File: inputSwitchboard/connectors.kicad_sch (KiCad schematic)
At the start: 0 parts

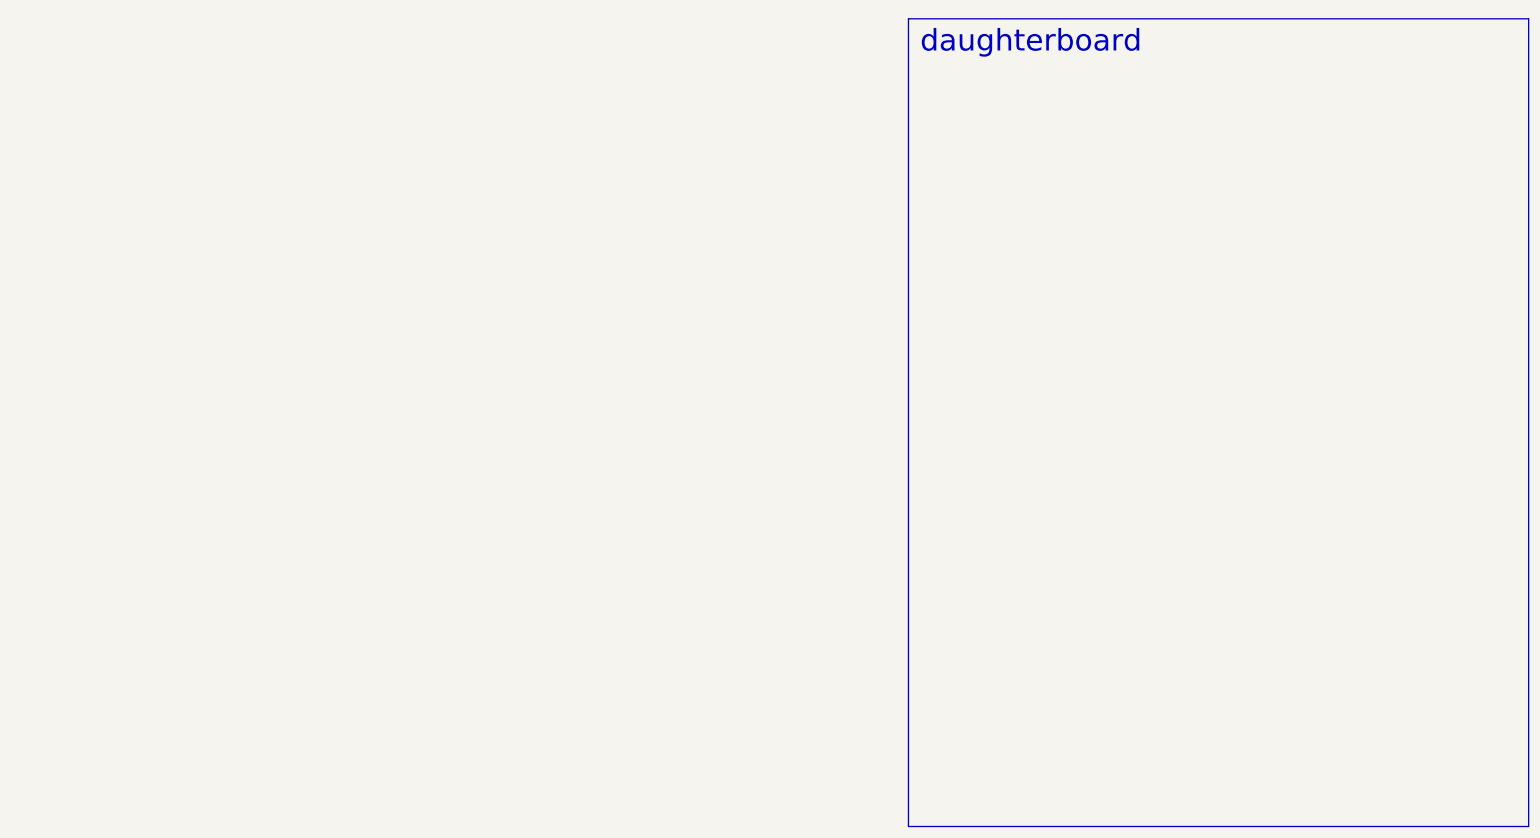
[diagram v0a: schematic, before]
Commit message: finished schematic
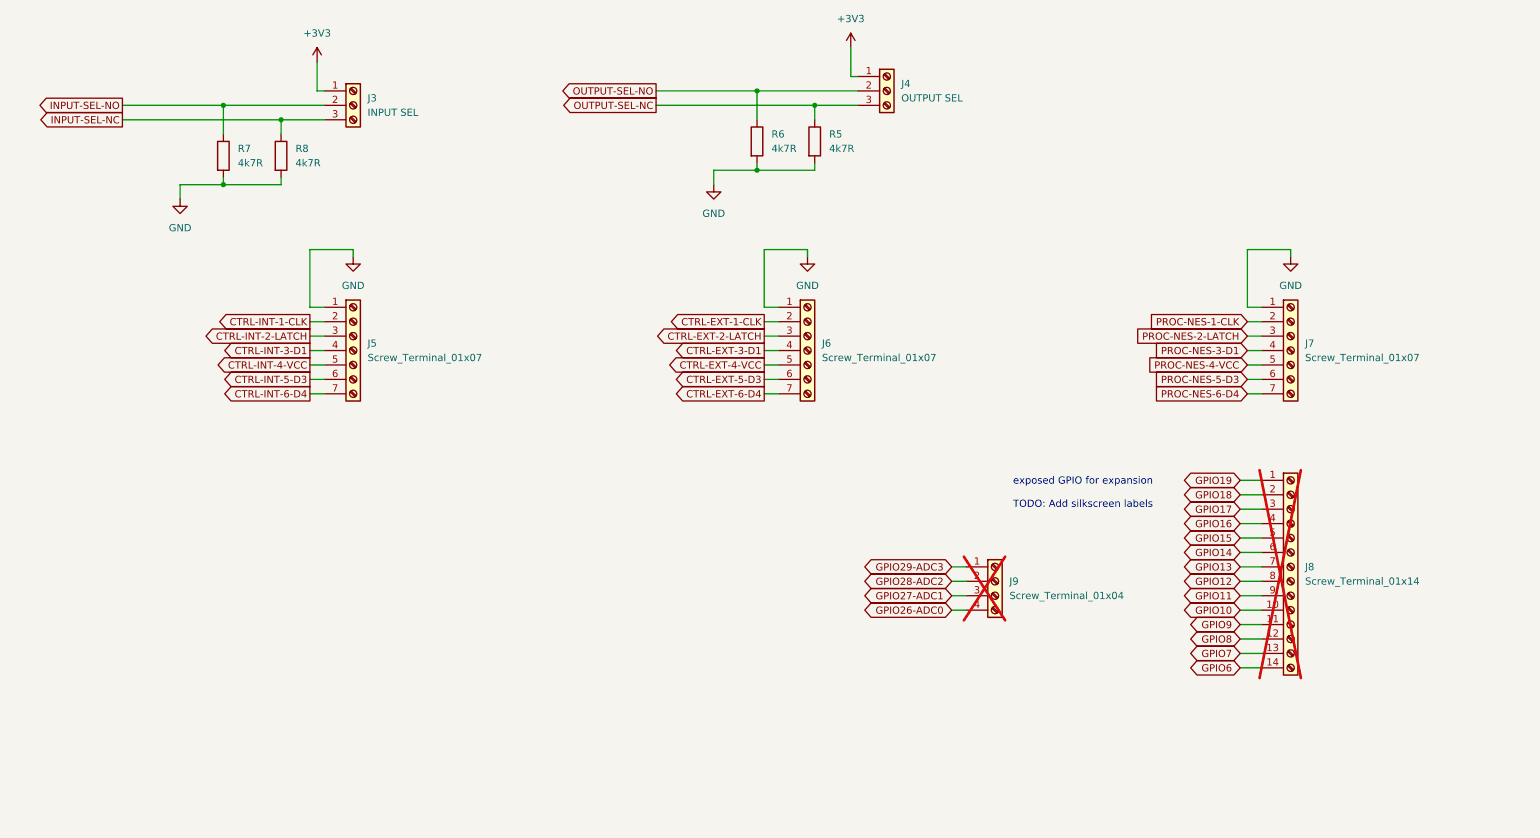
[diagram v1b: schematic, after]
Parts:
- added J3: INPUT SEL, TerminalBlock_Phoenix:TerminalBlock_Phoenix_MKDS-1,5-3-5.08_1x03_P5.08mm_Horizontal, symbol Connector:Screw_Terminal_01x03
- added J4: OUTPUT SEL, TerminalBlock_Phoenix:TerminalBlock_Phoenix_MKDS-1,5-3-5.08_1x03_P5.08mm_Horizontal, symbol Connector:Screw_Terminal_01x03
- added J5, J6, J7: Screw_Terminal_01x07, symbol Connector:Screw_Terminal_01x07
- added J8: Screw_Terminal_01x14, symbol Connector:Screw_Terminal_01x14
- added J9: Screw_Terminal_01x04, symbol Connector:Screw_Terminal_01x04
- added R5, R6, R7, R8: 4k7R, Resistor_SMD:R_0603_1608Metric, symbol Device:R
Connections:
- new net +3V3: J3.1 (Pin_1), J4.1 (Pin_1)
- new net CTRL-EXT-1-CLK: J6.2 (Pin_2)
- new net CTRL-EXT-2-LATCH: J6.3 (Pin_3)
- new net CTRL-EXT-3-D1: J6.4 (Pin_4)
- new net CTRL-EXT-4-VCC: J6.5 (Pin_5)
- new net CTRL-EXT-5-D3: J6.6 (Pin_6)
- new net CTRL-EXT-6-D4: J6.7 (Pin_7)
- new net CTRL-INT-1-CLK: J5.2 (Pin_2)
- new net CTRL-INT-2-LATCH: J5.3 (Pin_3)
- new net CTRL-INT-3-D1: J5.4 (Pin_4)
- new net CTRL-INT-4-VCC: J5.5 (Pin_5)
- new net CTRL-INT-5-D3: J5.6 (Pin_6)
- new net CTRL-INT-6-D4: J5.7 (Pin_7)
- new net GND: J5.1 (Pin_1), J6.1 (Pin_1), J7.1 (Pin_1), R5.2, R6.2, R7.2, R8.2
- new net GPIO10: J8.10 (Pin_10)
- new net GPIO11: J8.9 (Pin_9)
- new net GPIO12: J8.8 (Pin_8)
- new net GPIO13: J8.7 (Pin_7)
- new net GPIO14: J8.6 (Pin_6)
- new net GPIO15: J8.5 (Pin_5)
- new net GPIO16: J8.4 (Pin_4)
- new net GPIO17: J8.3 (Pin_3)
- new net GPIO18: J8.2 (Pin_2)
- new net GPIO19: J8.1 (Pin_1)
- new net GPIO26-ADC0: J9.4 (Pin_4)
- new net GPIO27-ADC1: J9.3 (Pin_3)
- new net GPIO28-ADC2: J9.2 (Pin_2)
- new net GPIO29-ADC3: J9.1 (Pin_1)
- new net GPIO6: J8.14 (Pin_14)
- new net GPIO7: J8.13 (Pin_13)
- new net GPIO8: J8.12 (Pin_12)
- new net GPIO9: J8.11 (Pin_11)
- new net INPUT-SEL-NC: J3.3 (Pin_3), R8.1
- new net INPUT-SEL-NO: J3.2 (Pin_2), R7.1
- new net OUTPUT-SEL-NC: J4.3 (Pin_3), R5.1
- new net OUTPUT-SEL-NO: J4.2 (Pin_2), R6.1
- new net PROC-NES-1-CLK: J7.2 (Pin_2)
- new net PROC-NES-2-LATCH: J7.3 (Pin_3)
- new net PROC-NES-3-D1: J7.4 (Pin_4)
- new net PROC-NES-4-VCC: J7.5 (Pin_5)
- new net PROC-NES-5-D3: J7.6 (Pin_6)
- new net PROC-NES-6-D4: J7.7 (Pin_7)
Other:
- note added: "exposed GPIO for expansion TODO: Add silkscreen labels"
- note removed: "daughterboard"
